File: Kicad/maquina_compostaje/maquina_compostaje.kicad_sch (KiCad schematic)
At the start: 0 parts

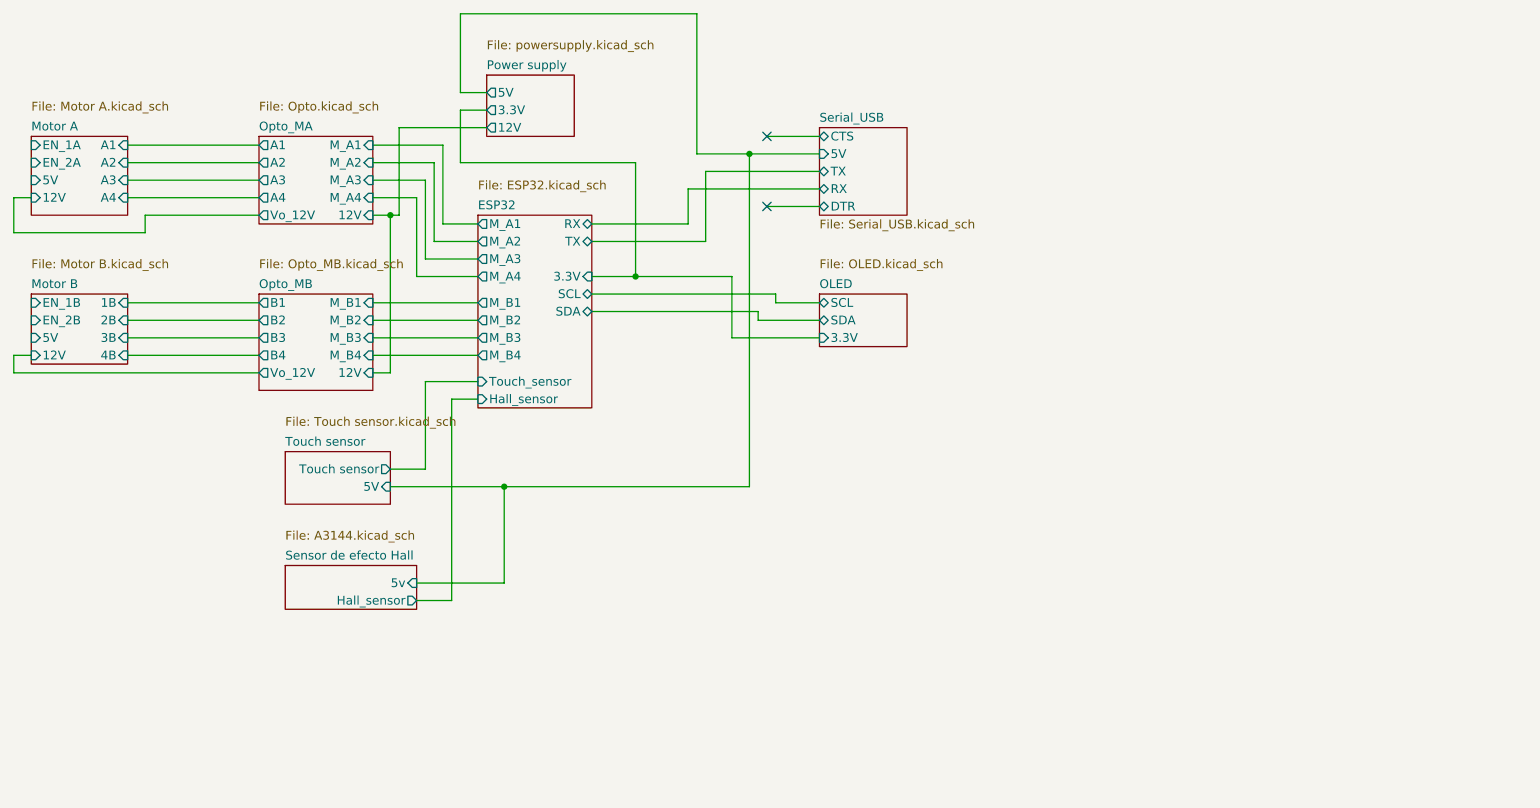
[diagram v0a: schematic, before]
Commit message: inicio del ruteo
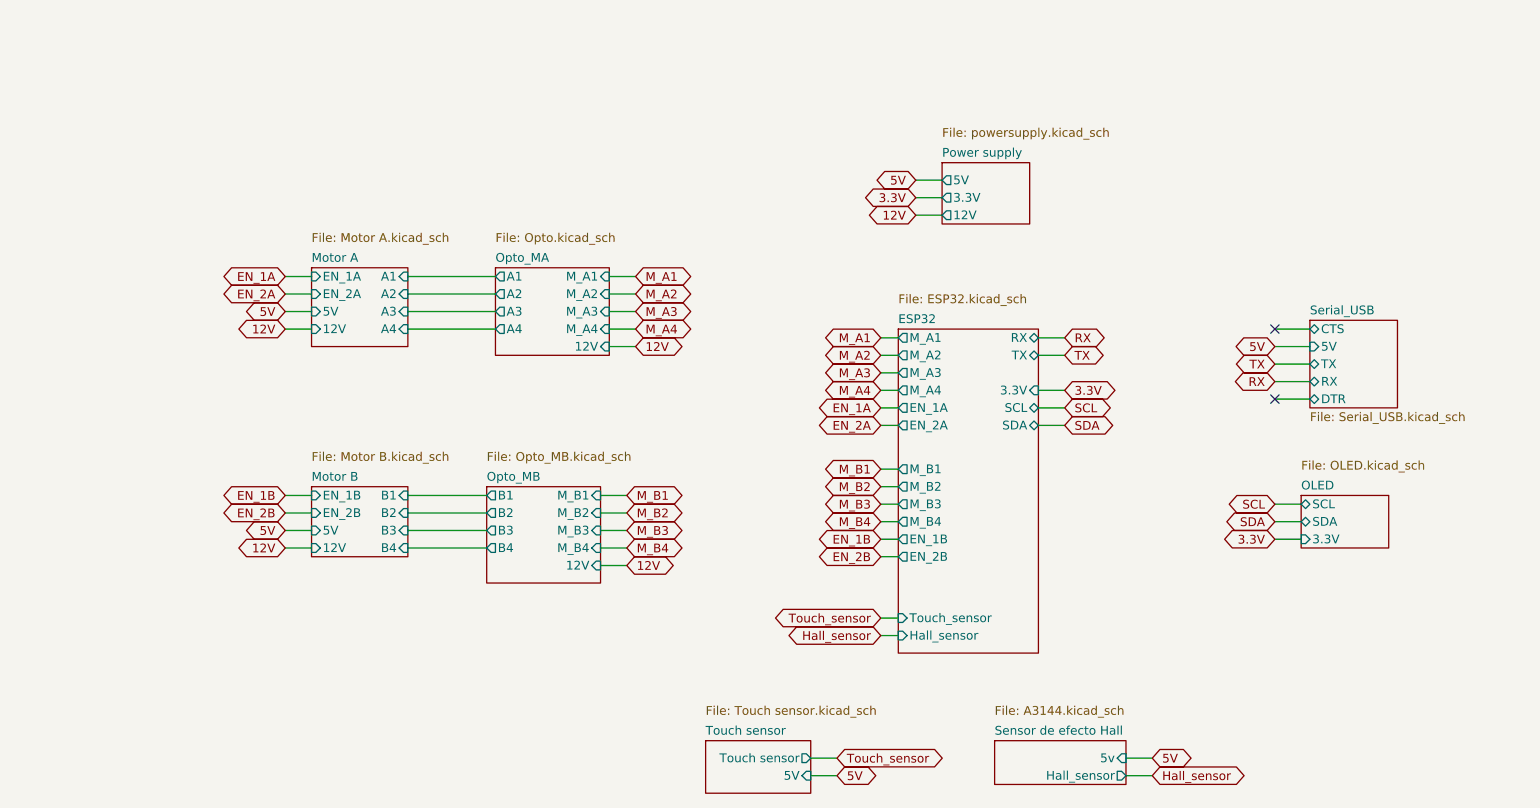
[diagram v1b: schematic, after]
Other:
- sheet ESP32 ports: added EN_1A, EN_1B, EN_2A, EN_2B; removed none
- sheet Motor B ports: added B1, B2, B3, B4; removed 1B, 2B, 3B, 4B
- sheet Opto_MA ports: added none; removed Vo_12V
- sheet Opto_MB ports: added none; removed Vo_12V
